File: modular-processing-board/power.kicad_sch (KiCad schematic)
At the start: 7 parts, among them J701 Conn_02x02_Odd_Even, U701 AMS1117-3.3

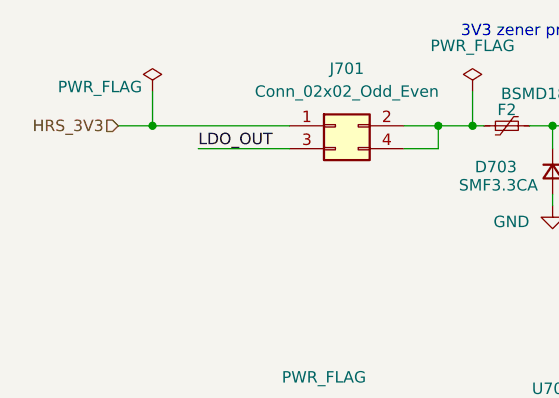
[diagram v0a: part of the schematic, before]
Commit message: figuring out delay matching for sdram
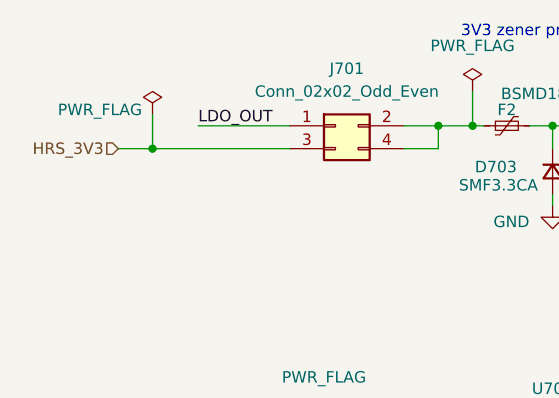
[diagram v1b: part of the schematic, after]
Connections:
- net HRS_3V3: now also J701.3 (Pin_3); no longer J701.1 (Pin_1)
- net LDO_OUT: now also J701.1 (Pin_1); no longer J701.3 (Pin_3)
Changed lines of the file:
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@@
 	)
 	(junction
-		(at 46.99 40.64)
+		(at 46.99 43.18)
 		(diameter 0)
 		(color 0 0 0 0)
@@
 	(wire
 		(pts
-			(xy 43.18 40.64) (xy 46.99 40.64)
-		)
-		(stroke
-			(width 0)
-			(type default)
-		)
-	)
-	(wire
-		(pts
 			(xy 120.65 40.64) (xy 125.73 40.64)
 		)
@@
 	(wire
 		(pts
-			(xy 46.99 36.83) (xy 46.99 40.64)
-		)
-		(stroke
-			(width 0)
-			(type default)
-		)
-	)
-	(wire
-		(pts
 			(xy 91.44 40.64) (xy 97.79 40.64)
 		)
@@
 	(wire
 		(pts
-			(xy 46.99 40.64) (xy 62.23 40.64)
-		)
-		(stroke
-			(width 0)
-			(type default)
-		)
-	)
-	(wire
-		(pts
 			(xy 105.41 40.64) (xy 113.03 40.64)
 		)
@@
 	(wire
 		(pts
-			(xy 52.07 43.18) (xy 62.23 43.18)
-		)
-		(stroke
-			(width 0)
-			(type default)
-		)
-	)
-	(wire
-		(pts
 			(xy 91.44 48.26) (xy 91.44 49.53)
 		)
@@
 	(wire
 		(pts
+			(xy 46.99 39.37) (xy 46.99 43.18)
+		)
+		(stroke
+			(width 0)
+			(type default)
+		)
+	)
+	(wire
+		(pts
 			(xy 100.33 40.64) (xy 100.33 43.18)
 		)
@@
 	(wire
 		(pts
+			(xy 52.07 40.64) (xy 62.23 40.64)
+		)
+		(stroke
+			(width 0)
+			(type default)
+		)
+	)
+	(wire
+		(pts
+			(xy 46.99 43.18) (xy 62.23 43.18)
+		)
+		(stroke
+			(width 0)
+			(type default)
+		)
+	)
+	(wire
+		(pts
 			(xy 100.33 40.64) (xy 105.41 40.64)
 		)
@@
 	(wire
 		(pts
+			(xy 43.18 43.18) (xy 46.99 43.18)
+		)
+		(stroke
+			(width 0)
+			(type default)
+		)
+	)
+	(wire
+		(pts
 			(xy 118.11 40.64) (xy 120.65 40.64)
 		)
@@
 			(width 0)
 			(type default)
+		)
+	)
+	(label "LDO_OUT"
+		(at 52.07 40.64 0)
+		(effects
+			(font
+				(size 1.27 1.27)
+			)
+			(justify left bottom)
 		)
 	)
@@
 		)
 	)
-	(label "LDO_OUT"
-		(at 52.07 43.18 0)
+	(hierarchical_label "USB_VBUS"
+		(shape input)
+		(at 62.23 76.2 180)
 		(effects
 			(font
 				(size 1.27 1.27)
 			)
-			(justify left bottom)
+			(justify right)
 		)
 	)
 	(hierarchical_label "HRS_3V3"
 		(shape input)
-		(at 43.18 40.64 180)
-		(effects
-			(font
-				(size 1.27 1.27)
-			)
-			(justify right)
-		)
-	)
-	(hierarchical_label "USB_VBUS"
-		(shape input)
-		(at 62.23 76.2 180)
+		(at 43.18 43.18 180)
 		(effects
 			(font
@@
 	(symbol
 		(lib_id "power:PWR_FLAG")
-		(at 46.99 36.83 0)
+		(at 46.99 39.37 0)
 		(unit 1)
 		(exclude_from_sim no)
@@
 		(dnp no)
 		(property "Reference" "#FLG0701"
-			(at 46.99 34.925 0)
+			(at 46.99 37.465 0)
 			(effects
 				(font
@@
 		)
 		(property "Value" "PWR_FLAG"
-			(at 41.148 36.322 0)
+			(at 41.148 38.862 0)
 			(effects
 				(font
@@
 		)
 		(property "Footprint" ""
-			(at 46.99 36.83 0)
+			(at 46.99 39.37 0)
 			(effects
 				(font
@@
 		)
 		(property "Datasheet" "~"
-			(at 46.99 36.83 0)
+			(at 46.99 39.37 0)
 			(effects
 				(font
@@
 		)
 		(property "Description" "Special symbol for telling ERC where power comes from"
-			(at 46.99 36.83 0)
-			(effects
-				(font
+			(at 46.99 39.37 0)
+			(effects
+				(font
